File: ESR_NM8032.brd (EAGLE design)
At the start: 34.9 x 90.8 mm, 79 parts, among them J1 0

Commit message: .
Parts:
- DA5: value 78l06 -> 78L06
- R15: value 2k4 -> 1k5(2k4 6v)
- R16: value 9k1 -> 7k5(9k1 6v)
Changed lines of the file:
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@@
 <layer number="35" name="tGlue" color="7" fill="4" visible="no" active="yes"/>
 <layer number="36" name="bGlue" color="7" fill="5" visible="no" active="yes"/>
-<layer number="37" name="tTest" color="7" fill="1" visible="no" active="yes"/>
-<layer number="38" name="bTest" color="7" fill="1" visible="no" active="yes"/>
+<layer number="37" name="tTest" color="7" fill="1" visible="yes" active="yes"/>
+<layer number="38" name="bTest" color="7" fill="1" visible="yes" active="yes"/>
 <layer number="39" name="tKeepout" color="4" fill="11" visible="no" active="yes"/>
 <layer number="40" name="bKeepout" color="1" fill="11" visible="no" active="yes"/>
@@
 <layer number="101" name="Patch_Top" color="12" fill="4" visible="yes" active="yes"/>
 <layer number="102" name="Vscore" color="7" fill="1" visible="yes" active="yes"/>
-<layer number="103" name="tMap" color="7" fill="1" visible="yes" active="yes"/>
-<layer number="104" name="Name" color="16" fill="1" visible="yes" active="yes"/>
+<layer number="103" name="tMap" color="7" fill="1" visible="no" active="yes"/>
+<layer number="104" name="Name" color="16" fill="1" visible="no" active="yes"/>
 <layer number="105" name="tPlate" color="7" fill="1" visible="yes" active="yes"/>
 <layer number="106" name="bPlate" color="7" fill="1" visible="yes" active="yes"/>
@@
 <layer number="114" name="bJumper" color="7" fill="1" visible="yes" active="yes"/>
 <layer number="115" name="GND" color="7" fill="1" visible="yes" active="yes"/>
-<layer number="116" name="Patch_BOT" color="9" fill="4" visible="yes" active="yes"/>
+<layer number="116" name="Patch_BOT" color="9" fill="4" visible="no" active="yes"/>
 <layer number="117" name="tJumper" color="9" fill="1" visible="yes" active="yes"/>
 <layer number="118" name="Rect_Pads" color="7" fill="1" visible="no" active="no"/>
+<layer number="119" name="119" color="7" fill="1" visible="yes" active="yes"/>
+<layer number="120" name="120" color="7" fill="1" visible="yes" active="yes"/>
 <layer number="121" name="_tsilk" color="7" fill="1" visible="yes" active="yes"/>
 <layer number="122" name="_bsilk" color="7" fill="1" visible="yes" active="yes"/>
@@
 <layer number="127" name="_tValues" color="7" fill="1" visible="yes" active="yes"/>
 <layer number="128" name="_bValues" color="7" fill="1" visible="yes" active="yes"/>
+<layer number="129" name="129" color="7" fill="1" visible="yes" active="yes"/>
+<layer number="130" name="130" color="7" fill="1" visible="no" active="yes"/>
 <layer number="131" name="tAdjust" color="7" fill="1" visible="yes" active="yes"/>
 <layer number="132" name="bAdjust" color="7" fill="1" visible="yes" active="yes"/>
+<layer number="133" name="133" color="7" fill="1" visible="no" active="yes"/>
 <layer number="144" name="Drill_legend" color="7" fill="1" visible="yes" active="yes"/>
 <layer number="150" name="Notes" color="7" fill="1" visible="yes" active="yes"/>
 <layer number="151" name="HeatSink" color="7" fill="1" visible="yes" active="yes"/>
-<layer number="152" name="_bDocu" color="7" fill="1" visible="yes" active="yes"/>
+<layer number="152" name="_bDocu" color="7" fill="1" visible="no" active="yes"/>
 <layer number="153" name="FabDoc1" color="7" fill="1" visible="yes" active="yes"/>
 <layer number="154" name="FabDoc2" color="7" fill="1" visible="yes" active="yes"/>
 <layer number="155" name="FabDoc3" color="7" fill="1" visible="yes" active="yes"/>
 <layer number="199" name="Contour" color="7" fill="1" visible="yes" active="yes"/>
-<layer number="200" name="200bmp" color="1" fill="10" visible="yes" active="yes"/>
-<layer number="201" name="201bmp" color="2" fill="10" visible="yes" active="yes"/>
-<layer number="202" name="202bmp" color="3" fill="10" visible="yes" active="yes"/>
-<layer number="203" name="203bmp" color="4" fill="10" visible="yes" active="yes"/>
-<layer number="204" name="204bmp" color="5" fill="10" visible="yes" active="yes"/>
-<layer number="205" name="205bmp" color="6" fill="10" visible="yes" active="yes"/>
-<layer number="206" name="206bmp" color="7" fill="10" visible="yes" active="yes"/>
-<layer number="207" name="207bmp" color="8" fill="10" visible="yes" active="yes"/>
-<layer number="208" name="208bmp" color="9" fill="10" visible="yes" active="yes"/>
+<layer number="200" name="200bmp" color="1" fill="10" visible="no" active="yes"/>
+<layer number="201" name="201bmp" color="2" fill="10" visible="no" active="yes"/>
+<layer number="202" name="202bmp" color="3" fill="10" visible="no" active="yes"/>
+<layer number="203" name="203bmp" color="4" fill="10" visible="no" active="yes"/>
+<layer number="204" name="204bmp" color="5" fill="10" visible="no" active="yes"/>
+<layer number="205" name="205bmp" color="6" fill="10" visible="no" active="yes"/>
+<layer number="206" name="206bmp" color="7" fill="10" visible="no" active="yes"/>
+<layer number="207" name="207bmp" color="8" fill="10" visible="no" active="yes"/>
+<layer number="208" name="208bmp" color="9" fill="10" visible="no" active="yes"/>
 <layer number="209" name="209bmp" color="7" fill="1" visible="yes" active="yes"/>
 <layer number="210" name="210bmp" color="7" fill="1" visible="yes" active="yes"/>
@@
 <attribute name="VALUE" x="20.32" y="87.63" size="1.27" layer="28" rot="MR90"/>
 </element>
-<element name="R16" library="rcl" package="M0805" value="9k1" x="22.225" y="96.8375" smashed="yes" rot="MR180">
+<element name="R16" library="rcl" package="M0805" value="7k5(9k1 6v)" x="22.225" y="96.8375" smashed="yes" rot="MR180">
 <attribute name="NAME" x="23.495" y="94.2975" size="1.27" layer="26" rot="MR0"/>
 <attribute name="VALUE" x="22.5425" y="93.6625" size="1.27" layer="28" rot="MR180"/>
 </element>
-<element name="R15" library="rcl" package="M0805" value="2k4" x="13.0175" y="96.8375" smashed="yes" rot="MR180">
+<element name="R15" library="rcl" package="M0805" value="1k5(2k4 6v)" x="13.0175" y="96.8375" smashed="yes" rot="MR180">
 <attribute name="NAME" x="11.1125" y="96.2025" size="1.27" layer="26" rot="MR0"/>
 <attribute name="VALUE" x="9.8425" y="90.805" size="1.27" layer="28" rot="MR90"/>
@@
 <attribute name="VALUE" x="10.795" y="50.546" size="1.27" layer="27" ratio="10"/>
 </element>
-<element name="DA5" library="ct-pack" package="SOT89R" value="78l06" x="7.62" y="72.0725" smashed="yes" rot="MR90">
+<element name="DA5" library="ct-pack" package="SOT89R" value="78L06" x="7.62" y="72.0725" smashed="yes" rot="MR90">
 <attribute name="NAME" x="10.1425" y="76.75" size="1.27" layer="26" rot="MR0"/>
 <attribute name="VALUE" x="10.7775" y="74.915" size="1.27" layer="28" rot="MR0"/>

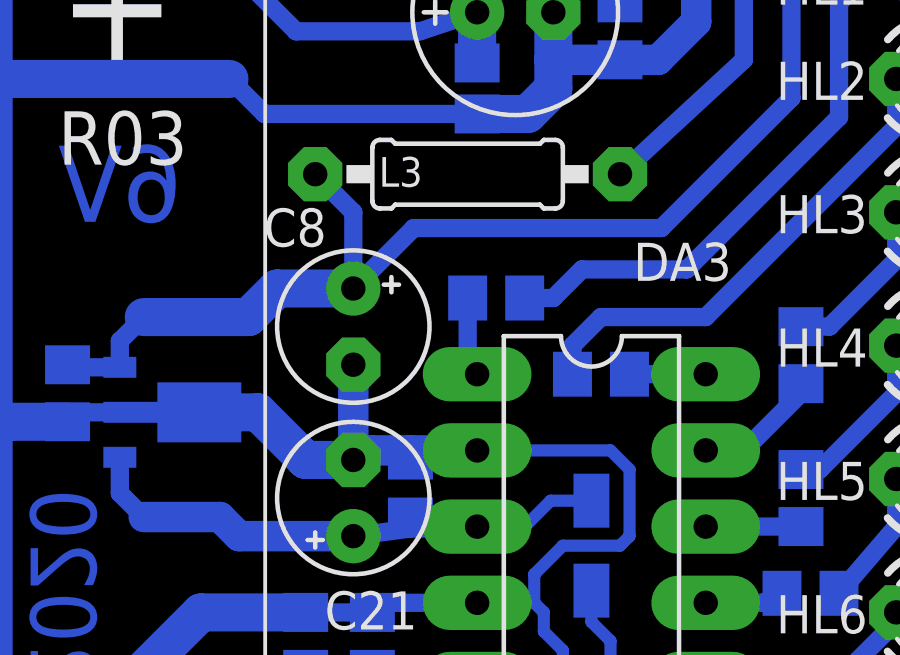
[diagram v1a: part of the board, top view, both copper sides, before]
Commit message: .
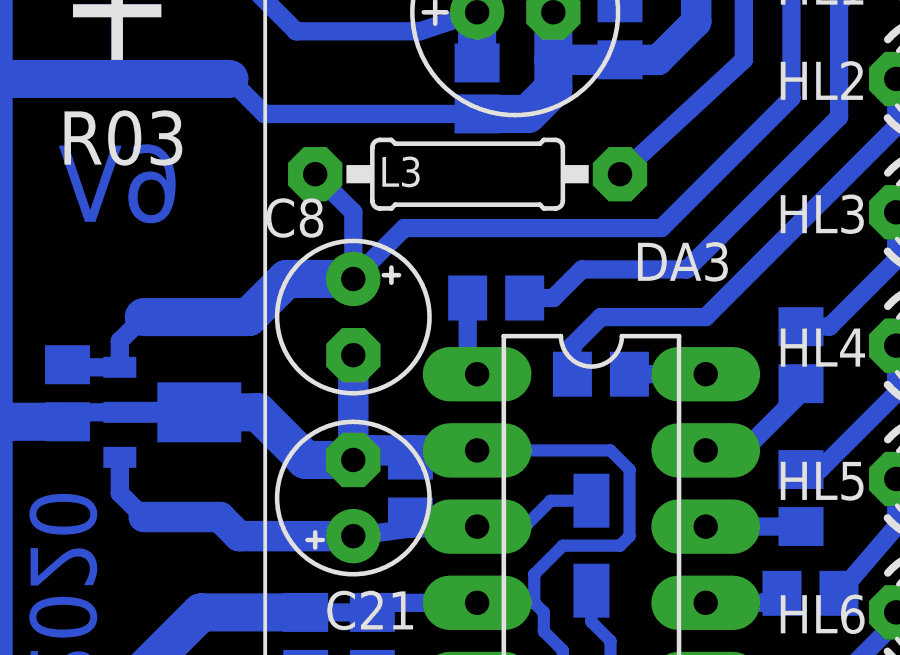
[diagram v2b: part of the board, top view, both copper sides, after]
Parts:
- moved C8 0.32 mm to (13.7, 75.2)
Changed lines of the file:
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@@
 <attribute name="VALUE" x="1.905" y="76.2" size="1.27" layer="28" rot="MR180"/>
 </element>
-<element name="C8" library="HWProgUSB" package="RCL_E2,5-5" value="100µ 16V" x="13.6525" y="74.93" smashed="yes" rot="R270">
-<attribute name="NAME" x="10.668" y="77.597" size="1.27" layer="25" ratio="10"/>
-<attribute name="VALUE" x="15.113" y="77.1525" size="1.27" layer="27" ratio="10"/>
+<element name="C8" library="HWProgUSB" package="RCL_E2,5-5" value="100µ 16V" x="13.6525" y="75.2475" smashed="yes" rot="R270">
+<attribute name="NAME" x="10.668" y="77.9145" size="1.27" layer="25" ratio="10"/>
+<attribute name="VALUE" x="15.113" y="77.47" size="1.27" layer="27" ratio="10"/>
 </element>
 <element name="U$1" library="ESR_NM8032" package="LR03" value="" x="5.715" y="30.1625" rot="R90"/>
@@
 <wire x1="8.52" y1="72.0725" x2="10.4775" y2="72.0725" width="1.27" layer="16"/>
 <wire x1="13.401" y1="70.4825" x2="13.6525" y2="70.485" width="1.016" layer="16"/>
-<wire x1="13.6525" y1="70.485" x2="13.6525" y2="73.66" width="1.016" layer="16"/>
-<wire x1="13.6525" y1="73.9775" x2="13.6525" y2="73.66" width="1.016" layer="16"/>
+<wire x1="13.6525" y1="70.485" x2="13.6525" y2="73.9775" width="1.016" layer="16"/>
 <wire x1="17.78" y1="70.8025" x2="15.5575" y2="70.8025" width="1.016" layer="16"/>
 <wire x1="15.5575" y1="70.8025" x2="14.224" y2="70.8025" width="1.016" layer="16"/>
@@
 <wire x1="4.2125" y1="73.5725" x2="4.1275" y2="73.6575" width="0.6096" layer="16"/>
 <contactref element="R17" pad="1"/>
-<wire x1="13.6525" y1="76.2" x2="11.1125" y2="76.2" width="1.27" layer="16"/>
-<wire x1="11.1125" y1="76.2" x2="10.16" y2="75.2475" width="1.27" layer="16"/>
+<wire x1="13.6525" y1="76.5175" x2="11.43" y2="76.5175" width="1.27" layer="16"/>
+<wire x1="11.43" y1="76.5175" x2="10.16" y2="75.2475" width="1.27" layer="16"/>
 <wire x1="10.16" y1="75.2475" x2="6.6675" y2="75.2475" width="1.27" layer="16"/>
 <wire x1="28.2575" y1="86.995" x2="28.2575" y2="82.55" width="0.6096" layer="16"/>
@@
 <wire x1="28.2575" y1="86.995" x2="31.4325" y2="90.17" width="0.6096" layer="16"/>
 <wire x1="31.4325" y1="90.17" x2="32.07" y2="90.17" width="0.6096" layer="16"/>
-<wire x1="13.6525" y1="76.2" x2="13.6525" y2="78.74" width="0.6096" layer="16"/>
+<wire x1="13.6525" y1="76.5175" x2="13.6525" y2="78.74" width="0.6096" layer="16"/>
 <wire x1="13.6525" y1="78.74" x2="12.3825" y2="80.01" width="0.6096" layer="16"/>
-<wire x1="23.921446875" y1="78.213946875" x2="15.666446875" y2="78.213946875" width="0.6096" layer="16"/>
-<wire x1="15.666446875" y1="78.213946875" x2="13.6525" y2="76.2" width="0.6096" layer="16"/>
+<wire x1="23.921446875" y1="78.213946875" x2="15.348946875" y2="78.213946875" width="0.6096" layer="16"/>
+<wire x1="15.348946875" y1="78.213946875" x2="13.6525" y2="76.5175" width="0.6096" layer="16"/>
 </signal>
 <signal name="+6V">
